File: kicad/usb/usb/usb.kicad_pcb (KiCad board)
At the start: 2 copper layers, 30 x 30 mm, 17 parts, among them J1 USB_C_Receptacle_USB2.0_14P, J2 PH2.0mm 2P, J3 Conn_01x07_Pin, SW1 PWR, U1 MCP73831-2-OT, U2 LW5233A23E, U3 HX809T-3.08V

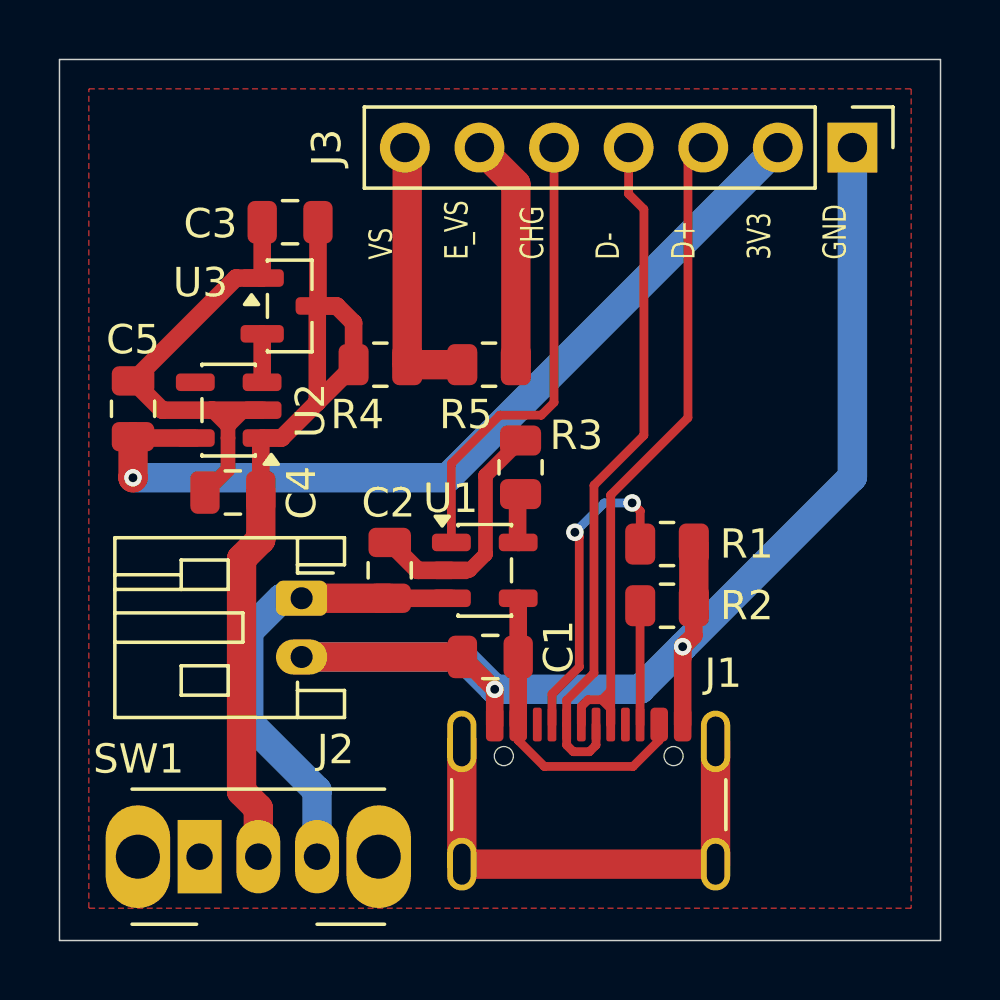
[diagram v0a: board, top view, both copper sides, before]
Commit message: Tons of changes regarding batteries...
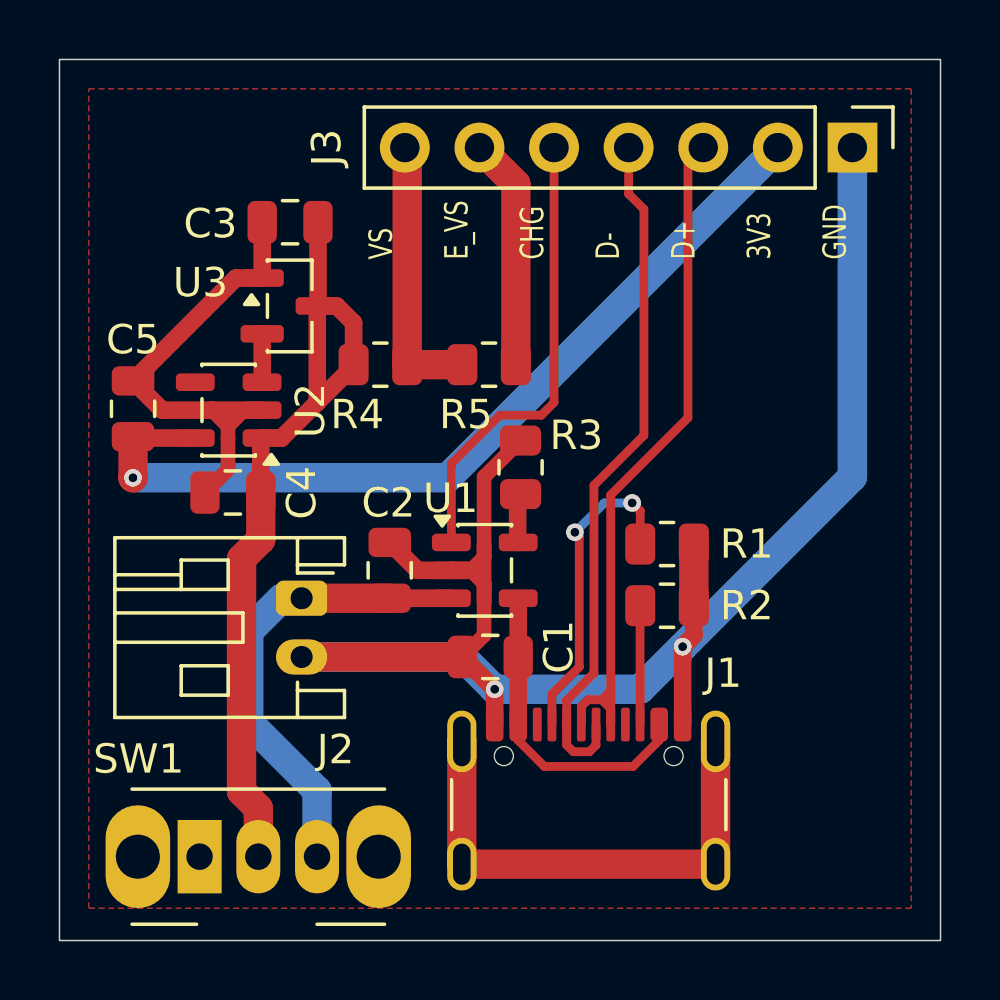
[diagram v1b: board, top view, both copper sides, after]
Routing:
- net GND: track 90.5 -> 95.9 mm
